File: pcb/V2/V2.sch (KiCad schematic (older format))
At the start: 46 parts, among them J1 Bat, J10 BatSw1, J11 BatSw2, J12 VideoV, J13 ServoV, J2 TSens+, J3 toFC, J4 Solar, J5 TSens-, J6 Heater1, J7 Heater2, J8 OC2, J9 OC1, M1 ACS712-5A, M2 Ads1115-Mod, M3 PCF8574_EbayMod, P1 MT3608, P2 MT3608, P3 MT3608, Q1 BC817-40, Q2 BC817-40, Q3 BC817-40, Q4 BC817-40, Q5 BC817-40, Q6 BC817-40, Q7 BC817-40, Q8 BC817-40, T1 AO4801A, T2 AO4801A, T3 AO4801A

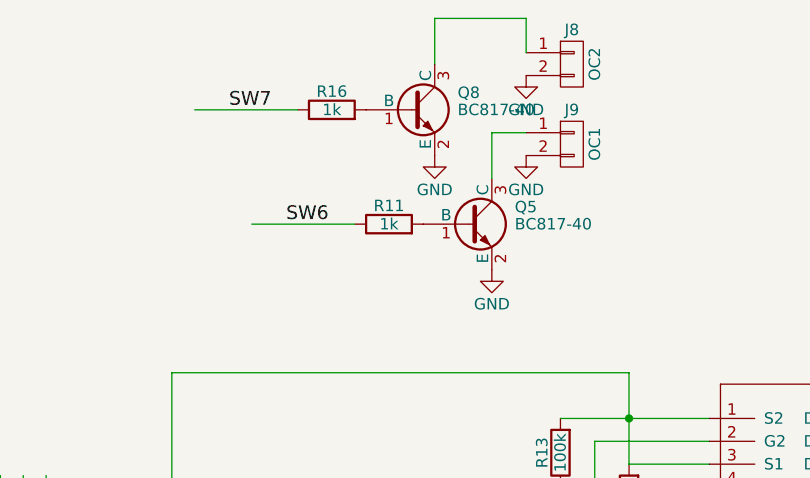
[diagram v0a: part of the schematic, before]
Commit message: Battery Management
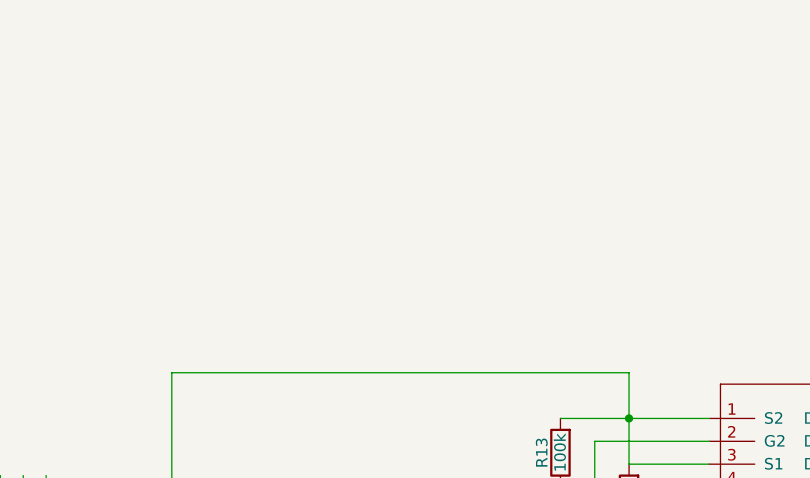
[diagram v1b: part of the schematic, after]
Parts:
- removed J8: OC2, symbol CONN_01X02
- removed J9: OC1, symbol CONN_01X02
- removed Q5, Q8: BC817-40, TO_SOT_Packages_SMD:SOT-23, symbol BC817-40
- removed R11, R16: 1k, Resistors_SMD:R_0603_HandSoldering, symbol R
- J1, J10, J11, J12, J13, J2, J4, J5, J6, J7: footprint (none) -> Pin_Headers:Pin_Header_Straight_1x02_Pitch2.54mm
- J3: footprint (none) -> Pin_Headers:Pin_Header_Straight_1x04_Pitch2.54mm
- M1: footprint (none) -> Franz-Mods:ACS712-Module
- M2: footprint (none) -> Franz-Mods:ADS1115-Module
- M3: footprint (none) -> Franz-Mods:PCF8574_Module
- P1, P2, P3: footprint Franz-Mods:MT3608 -> Franz-Mods:MT3608_module
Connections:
- wire segments 126 -> 119
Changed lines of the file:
@@
 F 0 "J1" H 1300 1500 50  0000 C CNN
 F 1 "Bat" V 1400 1350 50  0000 C CNN
-F 2 "" H 1300 1350 50  0001 C CNN
+F 2 "Pin_Headers:Pin_Header_Straight_1x02_Pitch2.54mm" H 1300 1350 50  0001 C CNN
 F 3 "" H 1300 1350 50  0001 C CNN
 	1    1300 1350
@@
 F 0 "M2" H 4100 2950 60  0000 C CNN
 F 1 "Ads1115-Mod" V 4200 3400 60  0000 C CNN
-F 2 "" H 3650 2750 60  0001 C CNN
+F 2 "Franz-Mods:ADS1115-Module" H 3650 2750 60  0001 C CNN
 F 3 "" H 3650 2750 60  0001 C CNN
 	1    3650 2750
@@
 F 0 "M1" H 2450 2700 60  0000 C CNN
 F 1 "ACS712-5A" H 2550 2850 60  0000 C CNN
-F 2 "" H 2100 2100 60  0001 C CNN
+F 2 "Franz-Mods:ACS712-Module" H 2100 2100 60  0001 C CNN
 F 3 "" H 2100 2100 60  0001 C CNN
 	1    2100 2100
@@
 F 0 "J3" H 5450 900 50  0000 C CNN
 F 1 "toFC" V 5550 650 50  0000 C CNN
-F 2 "" H 5450 650 50  0001 C CNN
+F 2 "Pin_Headers:Pin_Header_Straight_1x04_Pitch2.54mm" H 5450 650 50  0001 C CNN
 F 3 "" H 5450 650 50  0001 C CNN
 	1    5450 650
@@
 F 0 "J2" H 2950 3300 50  0000 C CNN
 F 1 "TSens+" V 3050 3150 50  0000 C CNN
-F 2 "" H 2950 3150 50  0001 C CNN
+F 2 "Pin_Headers:Pin_Header_Straight_1x02_Pitch2.54mm" H 2950 3150 50  0001 C CNN
 F 3 "" H 2950 3150 50  0001 C CNN
 F 4 "Value" H 2950 3150 60  0001 C CNN "Fieldname"
@@
 F 0 "P1" H 3000 5300 60  0000 C CNN
 F 1 "MT3608" H 3000 5550 60  0000 C CNN
-F 2 "Franz-Mods:MT3608" H 2800 5300 60  0001 C CNN
+F 2 "Franz-Mods:MT3608_module" H 2800 5300 60  0001 C CNN
 F 3 "" H 2800 5300 60  0001 C CNN
 	1    2800 5300
@@
 F 0 "J4" H 2000 4400 50  0000 C CNN
 F 1 "Solar" V 2100 4250 50  0000 C CNN
-F 2 "" H 2000 4250 50  0001 C CNN
+F 2 "Pin_Headers:Pin_Header_Straight_1x02_Pitch2.54mm" H 2000 4250 50  0001 C CNN
 F 3 "" H 2000 4250 50  0001 C CNN
 	1    2000 4250
@@
 F 0 "J5" H 2950 3750 50  0000 C CNN
 F 1 "TSens-" V 3050 3600 50  0000 C CNN
-F 2 "" H 2950 3600 50  0001 C CNN
+F 2 "Pin_Headers:Pin_Header_Straight_1x02_Pitch2.54mm" H 2950 3600 50  0001 C CNN
 F 3 "" H 2950 3600 50  0001 C CNN
 F 4 "Value" H 2950 3600 60  0001 C CNN "Fieldname"
@@
 F 0 "P2" H 10000 4450 60  0000 C CNN
 F 1 "MT3608" H 10000 4700 60  0000 C CNN
-F 2 "Franz-Mods:MT3608" H 9800 4450 60  0001 C CNN
+F 2 "Franz-Mods:MT3608_module" H 9800 4450 60  0001 C CNN
 F 3 "" H 9800 4450 60  0001 C CNN
 	1    9800 4450
@@
 F 0 "P3" H 10000 5000 60  0000 C CNN
 F 1 "MT3608" H 10000 5250 60  0000 C CNN
-F 2 "Franz-Mods:MT3608" H 9800 5000 60  0001 C CNN
+F 2 "Franz-Mods:MT3608_module" H 9800 5000 60  0001 C CNN
 F 3 "" H 9800 5000 60  0001 C CNN
 	1    9800 5000
@@
 F 0 "J13" H 10950 4300 50  0000 C CNN
 F 1 "ServoV" V 11050 4150 50  0000 C CNN
-F 2 "" H 10950 4150 50  0001 C CNN
+F 2 "Pin_Headers:Pin_Header_Straight_1x02_Pitch2.54mm" H 10950 4150 50  0001 C CNN
 F 3 "" H 10950 4150 50  0001 C CNN
 F 4 "Value" H 10950 4150 60  0001 C CNN "Fieldname"
@@
 F 0 "J12" H 10900 4850 50  0000 C CNN
 F 1 "VideoV" V 11000 4700 50  0000 C CNN
-F 2 "" H 10900 4700 50  0001 C CNN
+F 2 "Pin_Headers:Pin_Header_Straight_1x02_Pitch2.54mm" H 10900 4700 50  0001 C CNN
 F 3 "" H 10900 4700 50  0001 C CNN
 F 4 "Value" H 10900 4700 60  0001 C CNN "Fieldname"
@@
 F 0 "J6" H 7400 6150 50  0000 C CNN
 F 1 "Heater1" V 7500 6000 50  0000 C CNN
-F 2 "" H 7400 6000 50  0001 C CNN
+F 2 "Pin_Headers:Pin_Header_Straight_1x02_Pitch2.54mm" H 7400 6000 50  0001 C CNN
 F 3 "" H 7400 6000 50  0001 C CNN
 F 4 "Value" H 7400 6000 60  0001 C CNN "Fieldname"
@@
 F 0 "J7" H 7400 6550 50  0000 C CNN
 F 1 "Heater2" V 7500 6400 50  0000 C CNN
-F 2 "" H 7400 6400 50  0001 C CNN
+F 2 "Pin_Headers:Pin_Header_Straight_1x02_Pitch2.54mm" H 7400 6400 50  0001 C CNN
 F 3 "" H 7400 6400 50  0001 C CNN
 F 4 "Value" H 7400 6400 60  0001 C CNN "Fieldname"
@@
 F 0 "J10" H 10700 2450 50  0000 C CNN
 F 1 "BatSw1" V 10800 2300 50  0000 C CNN
-F 2 "" H 10700 2300 50  0001 C CNN
+F 2 "Pin_Headers:Pin_Header_Straight_1x02_Pitch2.54mm" H 10700 2300 50  0001 C CNN
 F 3 "" H 10700 2300 50  0001 C CNN
 F 4 "Value" H 10700 2300 60  0001 C CNN "Fieldname"
@@
 F 0 "J11" H 10700 2800 50  0000 C CNN
 F 1 "BatSw2" V 10800 2650 50  0000 C CNN
-F 2 "" H 10700 2650 50  0001 C CNN
+F 2 "Pin_Headers:Pin_Header_Straight_1x02_Pitch2.54mm" H 10700 2650 50  0001 C CNN
 F 3 "" H 10700 2650 50  0001 C CNN
 F 4 "Value" H 10700 2650 60  0001 C CNN "Fieldname"
@@
 $EndComp
 $Comp
-L GND #PWR030
-U 1 1 59C9EC25
-P 8250 1600
-F 0 "#PWR030" H 8250 1350 50  0001 C CNN
-F 1 "GND" H 8250 1450 50  0000 C CNN
-F 2 "" H 8250 1600 50  0001 C CNN
-F 3 "" H 8250 1600 50  0001 C CNN
-	1    8250 1600
-	1    0    0    -1
-$EndComp
-$Comp
-L R R11
-U 1 1 59C9EC2B
-P 7800 1400
-F 0 "R11" V 7880 1400 50  0000 C CNN
-F 1 "1k" V 7800 1400 50  0000 C CNN
-F 2 "Resistors_SMD:R_0603_HandSoldering" V 7730 1400 50  0001 C CNN
-F 3 "" H 7800 1400 50  0001 C CNN
-	1    7800 1400
-	0    -1   -1   0
-$EndComp
-Wire Wire Line
-	7650 1400 7200 1400
-$Comp
-L BC817-40 Q5
-U 1 1 59C9EC32
-P 8150 1400
-F 0 "Q5" H 8350 1475 50  0000 L CNN
-F 1 "BC817-40" H 8350 1400 50  0000 L CNN
-F 2 "TO_SOT_Packages_SMD:SOT-23" H 8350 1325 50  0001 L CIN
-F 3 "" H 8150 1400 50  0001 L CNN
-	1    8150 1400
-	1    0    0    -1
-$EndComp
-$Comp
-L CONN_01X02 J9
-U 1 1 59C9EE33
-P 8600 1050
-F 0 "J9" H 8600 1200 50  0000 C CNN
-F 1 "OC1" V 8700 1050 50  0000 C CNN
-F 2 "" H 8600 1050 50  0001 C CNN
-F 3 "" H 8600 1050 50  0001 C CNN
-F 4 "Value" H 8600 1050 60  0001 C CNN "Fieldname"
-	1    8600 1050
-	1    0    0    -1
-$EndComp
-$Comp
-L CONN_01X02 J8
-U 1 1 59C9EF12
-P 8600 700
-F 0 "J8" H 8600 850 50  0000 C CNN
-F 1 "OC2" V 8700 700 50  0000 C CNN
-F 2 "" H 8600 700 50  0001 C CNN
-F 3 "" H 8600 700 50  0001 C CNN
-F 4 "Value" H 8600 700 60  0001 C CNN "Fieldname"
-	1    8600 700
-	1    0    0    -1
-$EndComp
-Text Label 7350 1400 0    60   ~ 0
-SW6
-Wire Wire Line
-	8250 1200 8250 1000
-Wire Wire Line
-	8250 1000 8400 1000
-$Comp
-L GND #PWR031
-U 1 1 59C9F43B
-P 8400 1100
-F 0 "#PWR031" H 8400 850 50  0001 C CNN
-F 1 "GND" H 8400 950 50  0000 C CNN
-F 2 "" H 8400 1100 50  0001 C CNN
-F 3 "" H 8400 1100 50  0001 C CNN
-	1    8400 1100
-	1    0    0    -1
-$EndComp
-$Comp
-L GND #PWR032
-U 1 1 59C9F4CA
-P 8400 750
-F 0 "#PWR032" H 8400 500 50  0001 C CNN
-F 1 "GND" H 8400 600 50  0000 C CNN
-F 2 "" H 8400 750 50  0001 C CNN
-F 3 "" H 8400 750 50  0001 C CNN
-	1    8400 750
-	1    0    0    -1
-$EndComp
-$Comp
 L PCF8574_EbayMod M3
 U 1 1 59CA2BA9
@@
 F 0 "M3" H 5650 3050 60  0000 C CNN
 F 1 "PCF8574_EbayMod" H 5850 3250 60  0000 C CNN
-F 2 "" H 5700 3350 60  0001 C CNN
+F 2 "Franz-Mods:PCF8574_Module" H 5700 3350 60  0001 C CNN
 F 3 "" H 5700 3350 60  0001 C CNN
 	1    5700 3350
@@
 $EndComp
 $Comp
-L GND #PWR033
+L GND #PWR030
 U 1 1 59CA2F5C
 P 4950 3300
-F 0 "#PWR033" H 4950 3050 50  0001 C CNN
+F 0 "#PWR030" H 4950 3050 50  0001 C CNN
 F 1 "GND" H 4950 3150 50  0000 C CNN
 F 2 "" H 4950 3300 50  0001 C CNN
@@
 $EndComp
 $Comp
-L +5V #PWR034
+L +5V #PWR031
 U 1 1 59CA330D
 P 4950 3200
-F 0 "#PWR034" H 4950 3050 50  0001 C CNN
+F 0 "#PWR031" H 4950 3050 50  0001 C CNN
 F 1 "+5V" V 4950 3340 50  0000 C CNN
 F 2 "" H 4950 3200 50  0001 C CNN
@@
 Text Label 5600 2700 1    60   ~ 0
 SW7
-$Comp
-L GND #PWR035
-U 1 1 59CA45A8
-P 8000 1100
-F 0 "#PWR035" H 8000 850 50  0001 C CNN
-F 1 "GND" H 8000 950 50  0000 C CNN
-F 2 "" H 8000 1100 50  0001 C CNN
-F 3 "" H 8000 1100 50  0001 C CNN
-	1    8000 1100
-	1    0    0    -1
-$EndComp
-$Comp
-L R R16
-U 1 1 59CA45AE
-P 7550 900
-F 0 "R16" V 7630 900 50  0000 C CNN
-F 1 "1k" V 7550 900 50  0000 C CNN
-F 2 "Resistors_SMD:R_0603_HandSoldering" V 7480 900 50  0001 C CNN
-F 3 "" H 7550 900 50  0001 C CNN
-	1    7550 900
-	0    -1   -1   0
-$EndComp
-Wire Wire Line
-	7400 900  6950 900
-$Comp
-L BC817-40 Q8
-U 1 1 59CA45B5
-P 7900 900
-F 0 "Q8" H 8100 975 50  0000 L CNN
-F 1 "BC817-40" H 8100 900 50  0000 L CNN
-F 2 "TO_SOT_Packages_SMD:SOT-23" H 8100 825 50  0001 L CIN
-F 3 "" H 7900 900 50  0001 L CNN
-	1    7900 900
-	1    0    0    -1
-$EndComp
-Text Label 7100 900  0    60   ~ 0
-SW7
-Wire Wire Line
-	8000 700  8000 500
-Wire Wire Line
-	8000 500  8400 500
-Wire Wire Line
-	8400 500  8400 650
 $EndSCHEMATC
